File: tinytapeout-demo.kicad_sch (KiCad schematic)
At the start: 138 parts, among them J1 Conn_01x06, J12 613012243121, J13 613012243121, J14 613012243121, J15 USB4500-03-0-A_REVA, J16 2x20_P2.54mm_Pinheader, J17 Conn_01x03, J18 2x20_P2.54mm_Pinheader, J19 Conn_01x02, J2 Conn_01x04, J3 613012243121, J4 TT04_BREAKOUT_REVB, J5 613012243121, J6 613012243121, J7 Conn_01x02, J8 Conn_01x03, J9 Conn_01x24, Q1 DMN2005K, SW1 434121025816, SW2 434121025816, SW3 434121025816, SW4 418121270808, U1 157112V12700, U2 TLV1117LV33, U3 AP2112K-1.8, U4 74CBTLV3257, U7 W25Q32JVSS, X1 20MHz

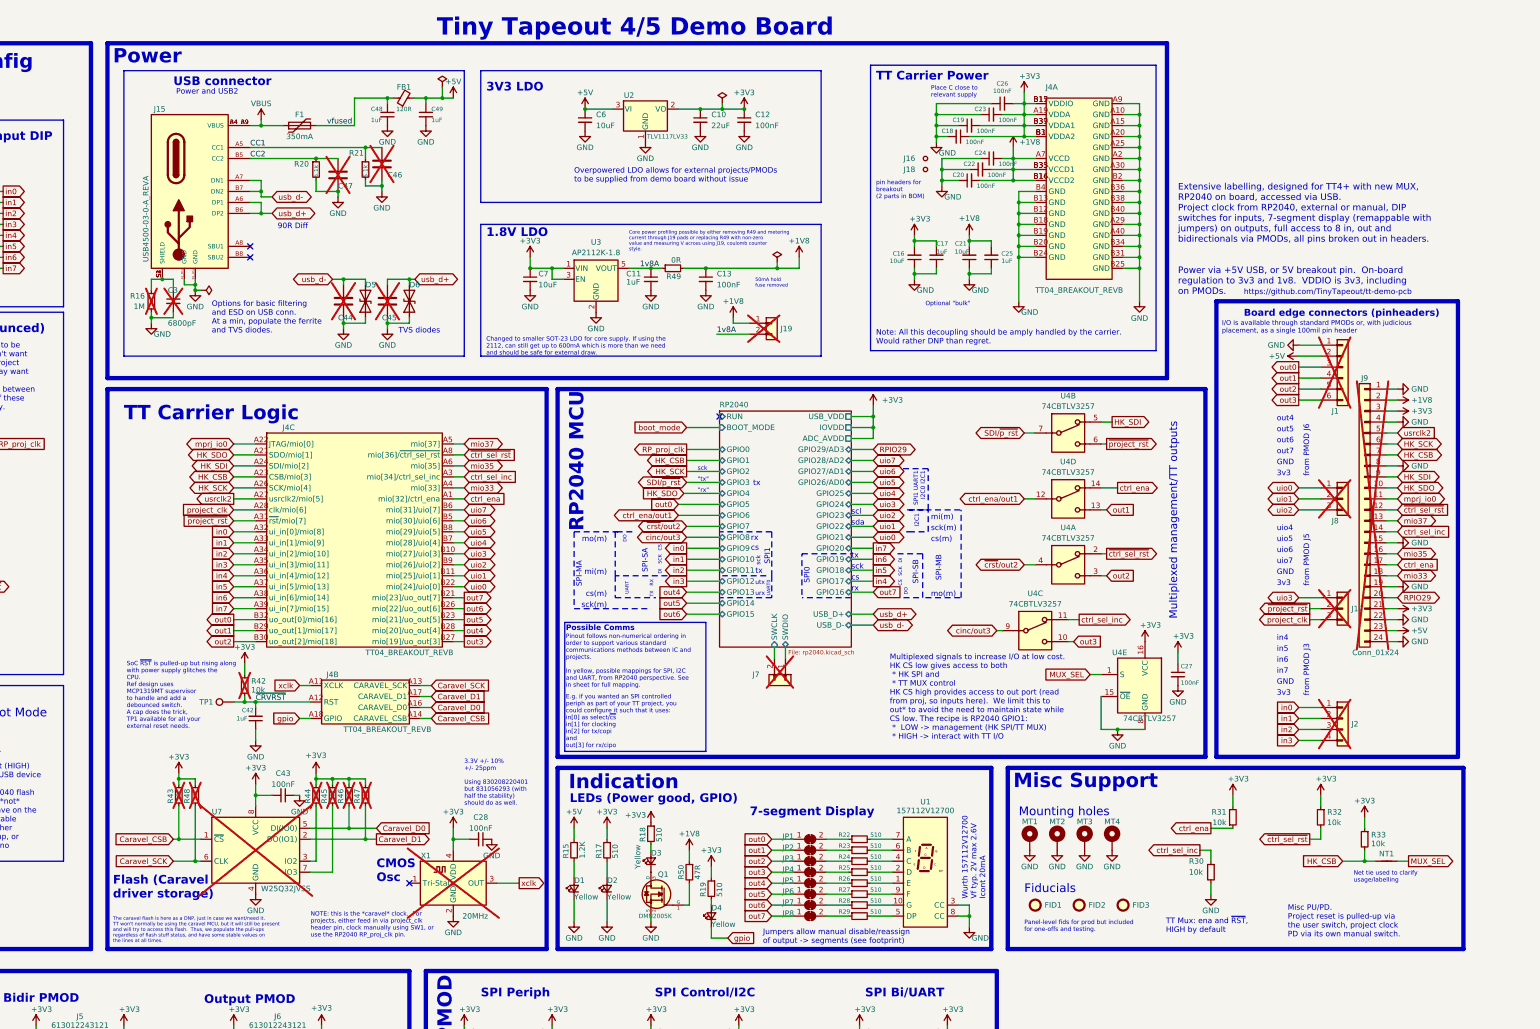
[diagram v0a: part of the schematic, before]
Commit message: TT06 prelim alpha1 schem
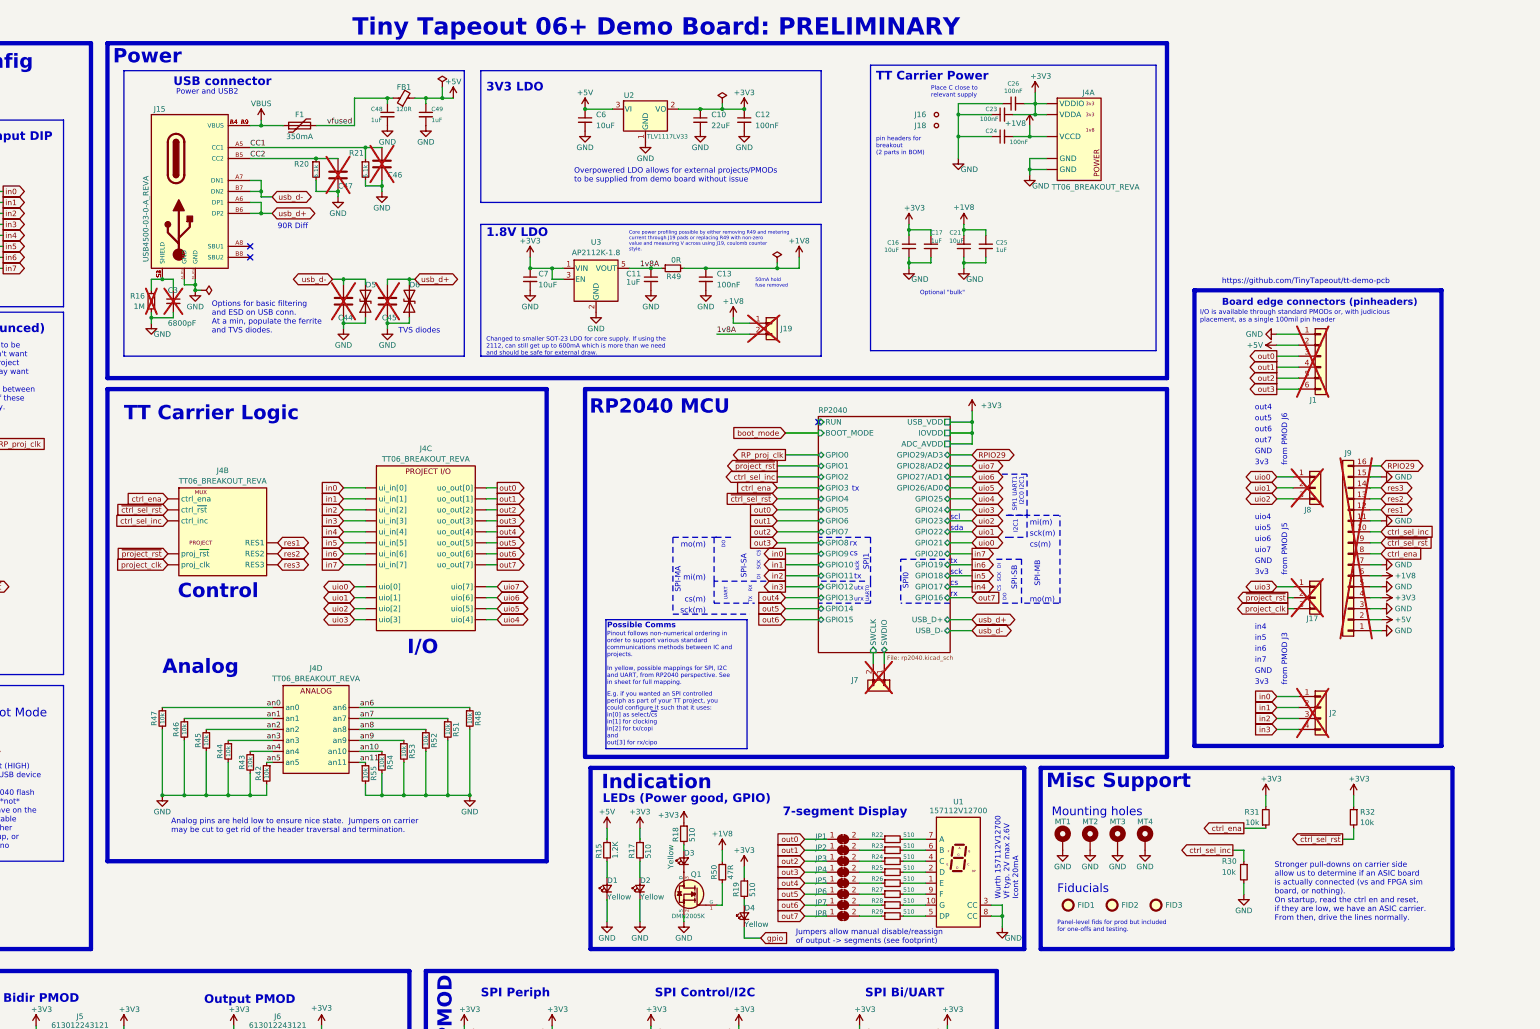
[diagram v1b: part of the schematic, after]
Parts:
- removed C18, C19, C20, C22, C27, C28, C43: 100nF, Capacitor_SMD:C_0402_1005Metric, symbol Device:C_Small
- removed C42: 1uF, Capacitor_SMD:C_0603_1608Metric, symbol Device:C_Small
- removed J4: TT04_BREAKOUT_REVB, TinyTapeout:TT04_BREAKOUT_SMB, symbol TinyTapeout:CARAVEL_TT04_BREAKOUT_REVB
- removed J9: Conn_01x24, Connector_PinHeader_2.54mm:PinHeader_1x24_P2.54mm_Vertical, symbol Connector_Generic:Conn_01x24
- removed NT1: NetTie_2, NetTie:NetTie-2_SMD_Pad0.5mm, symbol Device:NetTie_2
- removed R33: 10k, Resistor_SMD:R_0402_1005Metric, symbol Device:R_Small
- removed TP1: TestPoint, TestPoint:TestPoint_Pad_D1.5mm, symbol Connector:TestPoint
- removed U4: 74CBTLV3257, Package_SO:TSSOP-16_4.4x5mm_P0.65mm, symbol 74xx:74CBTLV3257
- removed U7: W25Q32JVSS, Package_SO:SOIC-8_5.23x5.23mm_P1.27mm, symbol Memory_Flash:W25Q32JVSS
- removed X1: 20MHz, Oscillator:Oscillator_SMD_ECS_2520MV-xxx-xx-4Pin_2.5x2.0mm, symbol Oscillator:ECS-2520MV-xxx-xx
- added J4: TT06_BREAKOUT_REVA, TinyTapeout:TT06_CARRIER_ON_DB, symbol TinyTapeout:OPENFRAME_TT06_BREAKOUT_REVA
- added J9: Conn_01x16, Connector_PinHeader_2.54mm:PinHeader_1x16_P2.54mm_Vertical, symbol Connector_Generic:Conn_01x16
- added R51, R52, R53, R54, R55: 10k, Resistor_SMD:R_0402_1005Metric, symbol Device:R_Small
- R42, R43, R44, R45, R46, R47, R48: now fitted
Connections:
- net Caravel_CSB is gone; now on net GND: R43.2
- net Caravel_D0 is gone; now on net GND: R46.2
- net Caravel_D1 is gone; now on net GND: R47.2
- net Caravel_SCK is gone; now on net GND: R48.2
- net ~{CRVRST} is gone; now on net GND: R42.2
- net +1V8: now also J4.A7 (VCCD), J9.6 (Pin_6)
- net +3V3: now also J4.B2 (VDDA), J4.B4 (VDDIO), J9.4 (Pin_4); no longer R42.1, R43.1, R44.1, R45.1, R46.1, R47.1, R48.1
- net +5V: now also J9.2 (Pin_2)
- net GND: now also R44.2, R45.2, J4.A1 (GND), J4.A12 (GND), J4.A15 (GND), J4.A18 (GND), J4.A21 (GND), J4.A23 (GND), J4.A25 (GND), J4.A27 (GND), J4.A29 (GND), J4.A31 (GND), J4.A32 (GND), J4.A33 (GND), J4.A37 (GND), J4.A38 (GND), J4.A5 (GND), J4.B1 (GND), J4.B10 (GND), J4.B12 (GND), J4.B14 (GND), J4.B16 (GND), J4.B17 (GND), J4.B18 (GND), J4.B23 (GND), J4.B24 (GND), J4.B29 (GND), J4.B3 (GND), J4.B30 (GND), J4.B35 (GND), J4.B36 (GND), J4.B39 (GND), J4.B40 (GND), J4.B6 (GND), J4.B8 (GND), J9.1 (Pin_1), J9.11 (Pin_11), J9.15 (Pin_15), J9.3 (Pin_3), J9.5 (Pin_5), J9.7 (Pin_7), R51.2, R52.2, R53.2, R54.2, R55.2
- net RPIO29: now also J9.16 (Pin_16)
- net ctrl_ena: now also J4.A2 (ctrl_ena), J9.8 (Pin_8)
- net ctrl_sel_inc: now also J4.A3 (ctrl_inc), J9.10 (Pin_10)
- net in0: now also J4.A9 (ui_in[0])
- net in1: now also J4.A11 (ui_in[1])
- net in2: now also J4.A14 (ui_in[2])
- net in3: now also J4.A13 (ui_in[3])
- net in4: now also J4.A17 (ui_in[4])
- net in5: now also J4.A19 (ui_in[5])
- net in6: now also J4.A16 (ui_in[6])
- net in7: now also J4.A34 (ui_in[7])
- net out0: now also J4.B27 (uo_out[0])
- net out1: now also J4.B28 (uo_out[1])
- net out2: now also J4.B25 (uo_out[2])
- net out3: now also J4.B26 (uo_out[3])
- net out4: now also J4.B21 (uo_out[4])
- net out5: now also J4.B22 (uo_out[5])
- net out6: now also J4.B19 (uo_out[6])
- net out7: now also J4.B20 (uo_out[7])
- net project_clk: now also J4.A35 (proj_clk)
- net uio0: now also J4.A39 (uio[0])
- net uio1: now also J4.A40 (uio[1])
- net uio2: now also J4.B37 (uio[2])
- net uio3: now also J4.B38 (uio[3])
- net uio4: now also J4.B33 (uio[4])
- net uio5: now also J4.B34 (uio[5])
- net uio6: now also J4.B31 (uio[6])
- net uio7: now also J4.B32 (uio[7])
- net ~{ctrl_sel_rst}: now also J4.A4 (ctrl_~{rst}), J9.9 (Pin_9)
- net ~{project_rst}: now also J4.A36 (proj_~{rst})
- new net an0: J4.A20 (an0), R47.1
- new net an1: J4.A22 (an1), R46.1
- new net an10: J4.B7 (an10), R54.1
- new net an11: J4.B5 (an11), R55.1
- new net an2: J4.A24 (an2), R45.1
- new net an3: J4.A26 (an3), R44.1
- new net an4: J4.A28 (an4), R43.1
- new net an5: J4.A30 (an5), R42.1
- new net an6: J4.B15 (an6), R48.1
- new net an7: J4.B13 (an7), R51.1
- new net an8: J4.B11 (an8), R52.1
- new net an9: J4.B9 (an9), R53.1
- new net res1: J4.A6 (RES1), J9.12 (Pin_12)
- new net res2: J4.A8 (RES2), J9.13 (Pin_13)
- new net res3: J4.A10 (RES3), J9.14 (Pin_14)
- no-connect marks 4 -> 3
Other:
- note added: "Analog"
- note added: "Analog pins are held low to ensure nice state. Jumpers on carrier may be cut to get rid of the header traversal and termination."
- note added: "Control"
- note added: "I/O"
- note added: "Stronger pull-downs on carrier side allow us to determine if an ASIC board is actually connected (vs and FPGA sim board, or nothing). On startup, read the ctrl en and reset, if they are low, we have an ASIC carrier. From then, drive the lines normally."
- note added: "Tiny Tapeout 06+ Demo Board: PRELIMINARY"
- note removed: ""rx""
- note removed: ""tx""
- note removed: "3.3V +/- 10% +/- 25ppm Using 830208220401 but 831056293 (with half the stability) should do as well."
- note removed: "CMOS Osc"
- note removed: "Extensive labelling, designed for TT4+ with new MUX, RP2040 on board, accessed via USB. Project clock from RP2040, external or manual, DIP switches for inputs, 7-segment display (remappable with jumpers) on outputs, full access to 8 in, out and bidirectionals via PMODs, all pins broken out in headers. Power via +5V USB, or 5V breakout pin. On-board regulation to 3v3 and 1v8. VDDIO is 3v3, includi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"
- note removed: "Flash (Caravel driver storage)"
- note removed: "Misc PU/PD. Project reset is pulled-up via the user switch, project clock PD via its own manual switch."
- note removed: "Multiplexed management/TT outputs"
- note removed: "Multiplexed signals to increase I/O at low cost. HK CS low gives access to both * HK SPI and * TT MUX control HK CS high provides access to out port (read from proj, so inputs here). We limit this to out* to avoid the need to maintain state while CS low. The recipe is RP2040 GPIO1: * LOW -> management (HK SPI/TT MUX) * HIGH -> interact with TT I/O"
- note removed: "NOTE: this is the *caravel* clock. For projects, either feed in via project_clk header pin, clock manually using SW1, or use the RP2040 RP_proj_clk pin."
- note removed: "Net tie used to clarify usage/labelling"
- note removed: "Note: All this decoupling should be amply handled by the carrier. Would rather DNP than regret."
- note removed: "SoC ~{RST} is pulled-up but rising along with power supply glitches the CPU. Ref design uses MCP1319MT supervisor to handle and add a debounced switch. A cap does the trick, TP1 available for all your external reset needs."
- note removed: "TT Mux: ena and ~{RST}, HIGH by default"
- note removed: "The caravel flash is here as a DNP, just in case we want/need it. TT won't normally be using the caravel MCU, but it will still be present and will try to access this flash. Thus, we populate the pull-ups regardless of flash stuff status, and have some stable values on the lines at all times."
- note removed: "Tiny Tapeout 4/5 Demo Board"
- moved on the sheet: C16, C17, C21, C23, C24, C25, C26, D1, D2, D3, D4, FID1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
